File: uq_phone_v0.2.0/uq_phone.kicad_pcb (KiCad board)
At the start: 4 copper layers, 42.8 x 103.8 mm, 146 parts, among them J1 USB4105-GF-A, J10 SJ-3551B-MSMT-TR-67, J11 Conn_01x02, J2 BM03B-ACHSS-GAN-TF_LF__SN_, J3 20279-001E-03, J4 20279-001E-03, J5 6871XX14022_68715014022, J6 Conn_ARM_SWD_TagConnect_TC2030, J7 Conn_01x02, J8 KP15B-6S-SF_800_, M1 VCDM0834B004L, Q1 MMBT3904LP-7, Q2 MMBT3904LP-7, U1 MCP73871-2CCI_ML, U10 TPD3F303DQDR, U11 TPD8F003DQDR, U12 MCP1664T-E/OT, U13 TS3A5018RSVR, U14 NAU88C22YG, U2 TPS62162DSGR, U3 BQ27441DRZR-G1A, U4 WP SNAP-IN BASE_6000636, U5 TXB0108RGYR, U6 TXB0108RGYR, U7 STM32H733VGTx, U8 LSM6DSVTR, U9 DRV2603RUNR

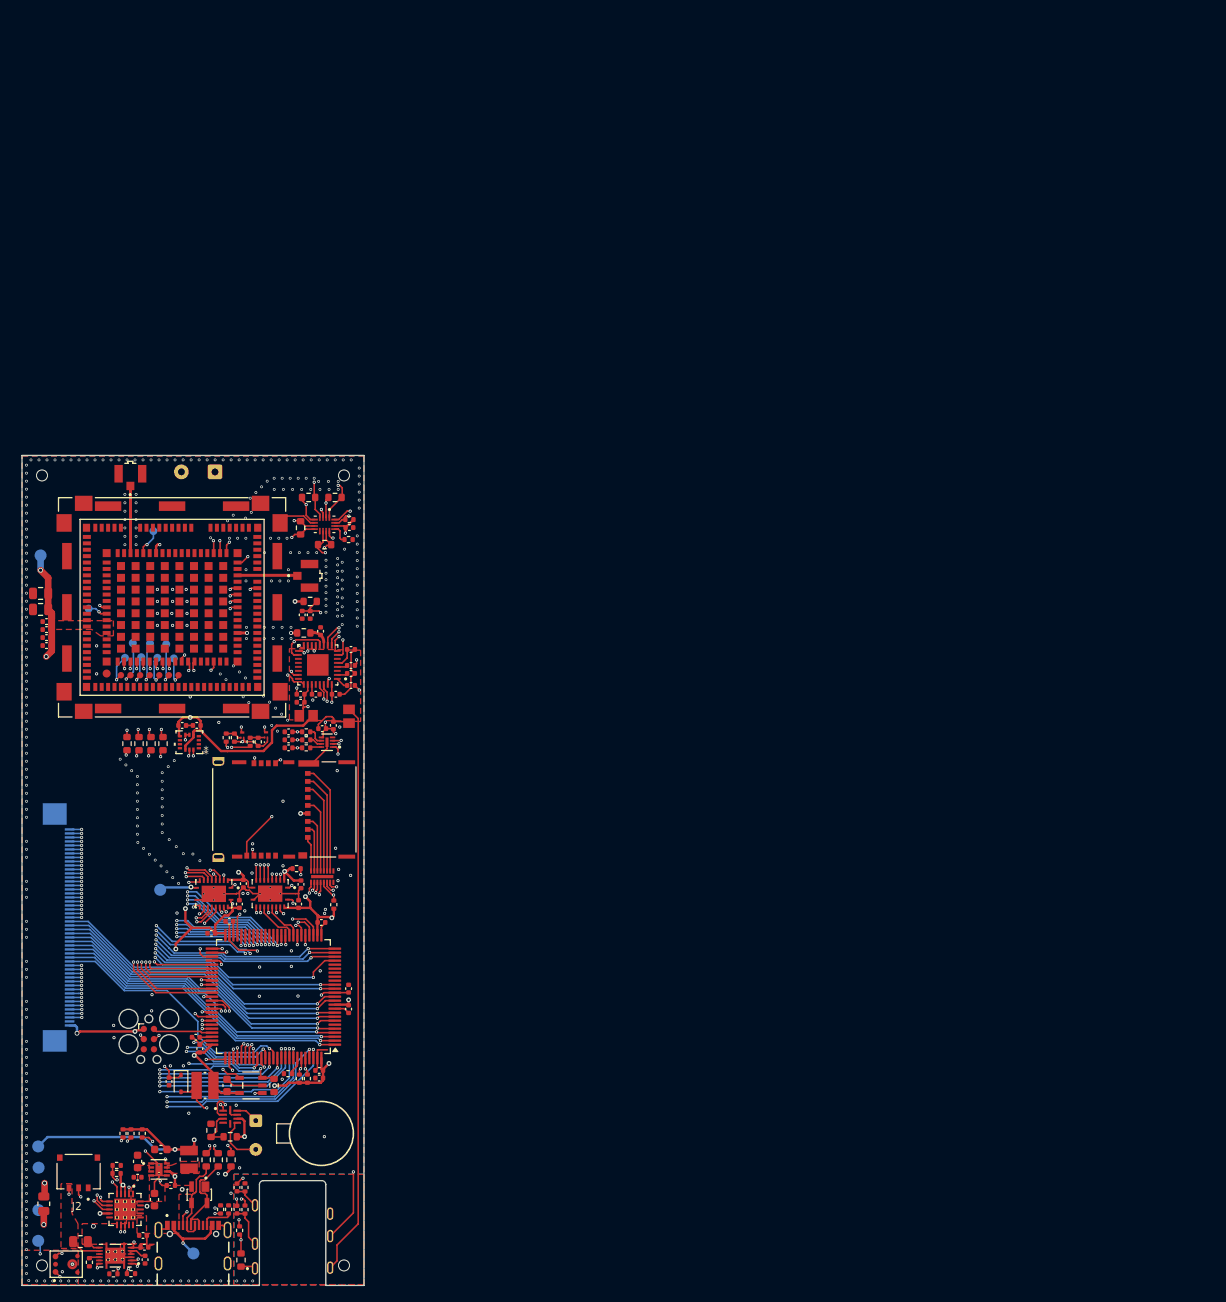
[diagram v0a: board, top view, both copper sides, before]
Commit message: Clean repo
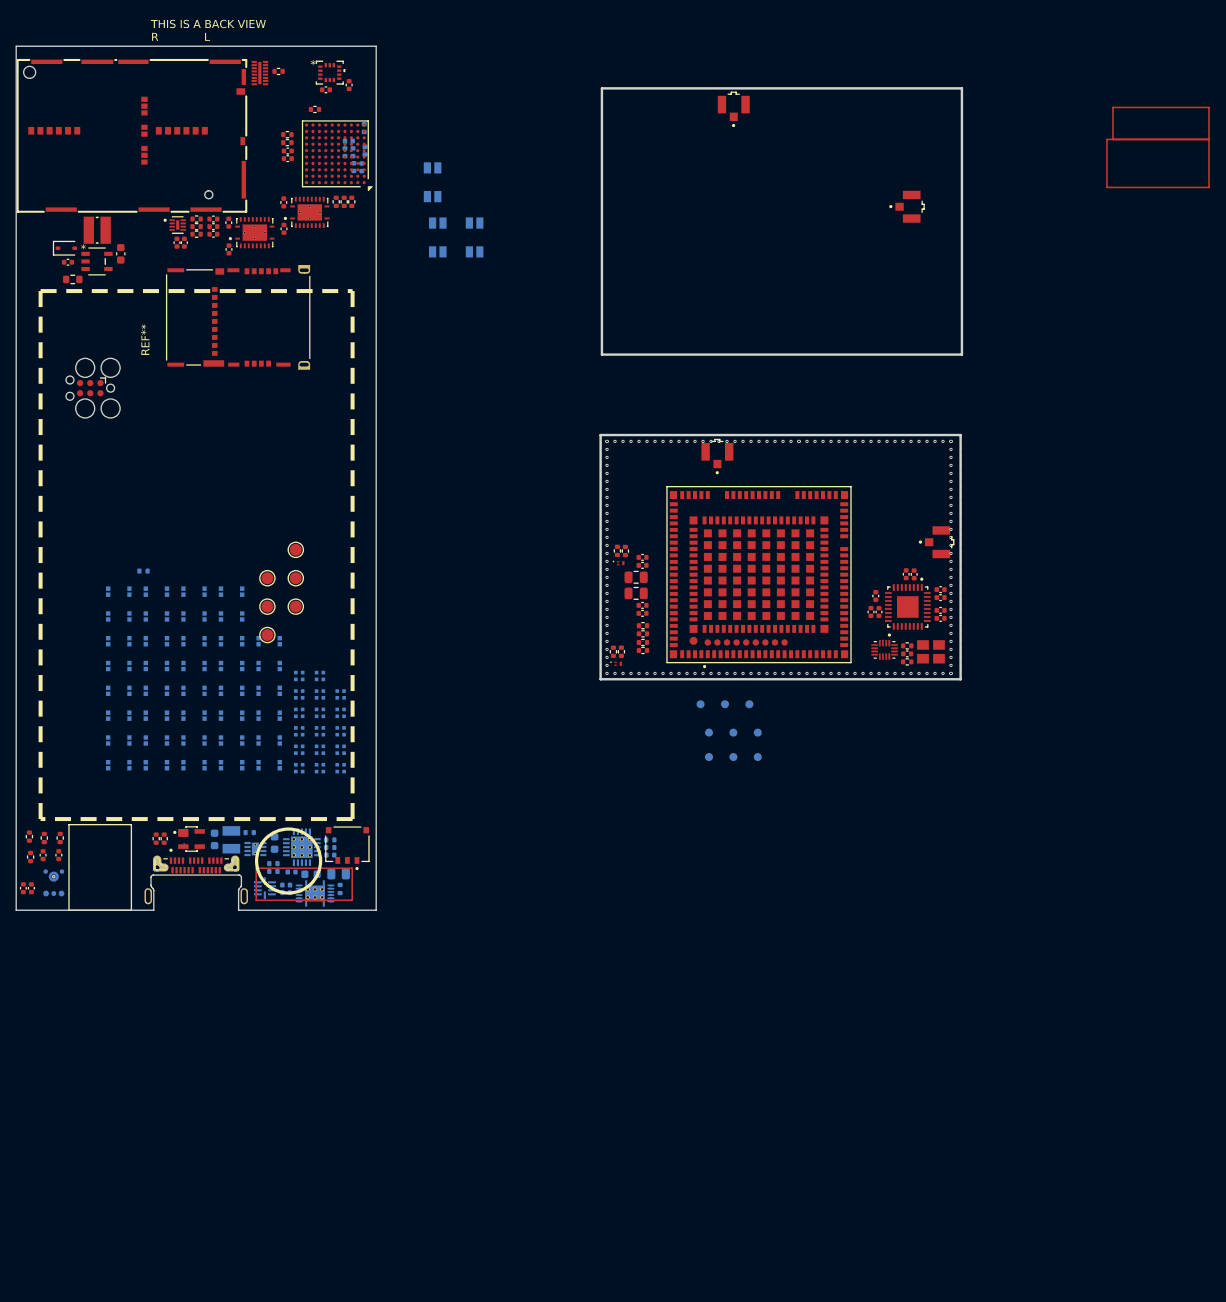
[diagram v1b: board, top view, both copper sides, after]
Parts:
- removed J1: USB4105-GF-A, USB_C_connector:GCT_USB4105-GF-A
- removed J10: SJ-3551B-MSMT-TR-67, SJ-3551B-MSMT-TR-67:CUI_SJ-3551B-MSMT-TR-67
- removed J11: Conn_01x02, Connector_Wire:SolderWire-0.25sqmm_1x02_P4.2mm_D0.65mm_OD1.7mm
- removed the J4 at (63.3, 83.3)
- removed the J5 at (31.0, 127.2)
- removed J7: Conn_01x02, Connector_Wire:SolderWire-0.1sqmm_1x02_P3.6mm_D0.4mm_OD1mm
- removed M1: VCDM0834B004L, custom_footprints:Motor_8mm
- removed R30, R31: 22R, Resistor_SMD:R_0402_1005Metric
- removed R34: 3.83R, Resistor_SMD:R_0603_1608Metric
- removed R35, R44, R49: 10k, Resistor_SMD:R_0402_1005Metric
- removed R37, R41, R43, R46, R47: 0R, Resistor_SMD:R_0603_1608Metric
- removed R4: 100k, Resistor_SMD:R_0402_1005Metric
- removed R45: 47k, Resistor_SMD:R_0402_1005Metric
- removed TP1: TestPoint, TestPoint:TestPoint_Pad_D1.5mm
- added J4: 20279-001E-03, 20279-001E-03:IPEX_20279-001E-03, F.Cu at (116.3, 24.4)
- added J4: 20279-001E-03, 20279-001E-03:IPEX_20279-001E-03, F.Cu at (114.3, 67.8)
- added J5: 20279-001E-03, 20279-001E-03:IPEX_20279-001E-03, F.Cu at (138.6, 37.2)
- added J5: 20279-001E-03, 20279-001E-03:IPEX_20279-001E-03, F.Cu at (142.3, 79.1)
- added LED1: XL-1010RGBC, custom_footprints:XL-1010RGBC-WS2812B, B.Cu at (62.0, 107.3)
- added LED10: XL-1010RGBC, custom_footprints:XL-1010RGBC-WS2812B, B.Cu at (64.6, 100.4)
- added LED11: XL-1010RGBC, custom_footprints:XL-1010RGBC-WS2812B, B.Cu at (64.6, 98.1)
- added LED12: XL-1010RGBC, custom_footprints:XL-1010RGBC-WS2812B, B.Cu at (64.6, 95.8)
- added LED13: XL-1010RGBC, custom_footprints:XL-1010RGBC-WS2812B, B.Cu at (67.2, 107.3)
- added LED14: XL-1010RGBC, custom_footprints:XL-1010RGBC-WS2812B, B.Cu at (67.2, 105.0)
- added LED15: XL-1010RGBC, custom_footprints:XL-1010RGBC-WS2812B, B.Cu at (67.2, 102.7)
- added LED16: XL-1010RGBC, custom_footprints:XL-1010RGBC-WS2812B, B.Cu at (67.2, 100.4)
- added LED17: XL-1010RGBC, custom_footprints:XL-1010RGBC-WS2812B, B.Cu at (67.2, 98.1)
- added LED2: XL-1010RGBC, custom_footprints:XL-1010RGBC-WS2812B, B.Cu at (62.0, 105.0)
- added LED3: XL-1010RGBC, custom_footprints:XL-1010RGBC-WS2812B, B.Cu at (62.0, 102.7)
- added LED4: XL-1010RGBC, custom_footprints:XL-1010RGBC-WS2812B, B.Cu at (62.0, 100.4)
- added LED5: XL-1010RGBC, custom_footprints:XL-1010RGBC-WS2812B, B.Cu at (62.0, 98.1)
- added LED6: XL-1010RGBC, custom_footprints:XL-1010RGBC-WS2812B, B.Cu at (62.0, 95.8)
- added LED7: XL-1010RGBC, custom_footprints:XL-1010RGBC-WS2812B, B.Cu at (64.6, 107.3)
- added LED8: XL-1010RGBC, custom_footprints:XL-1010RGBC-WS2812B, B.Cu at (64.6, 105.0)
- added LED9: XL-1010RGBC, custom_footprints:XL-1010RGBC-WS2812B, B.Cu at (64.6, 102.7)
- added R23: 10k, Resistor_SMD:R_0402_1005Metric, F.Cu at (60.5, 28.1)
- added REF**: HIROSE_KP15B-6S-SF_800_, KP15B-6S-SF_800_:HIROSE_KP15B-6S-SF_800_, F.Cu at (54.4, 51.0)
- added SW1: SKTAAAE010, custom_footprints:SKTAAAE010, B.Cu at (39.5, 107.0)
- added SW10: SKTAAAE010, custom_footprints:SKTAAAE010, B.Cu at (44.1, 107.0)
- added SW11: SKTAAAE010, custom_footprints:SKTAAAE010, B.Cu at (44.1, 103.8)
- added SW12: SKTAAAE010, custom_footprints:SKTAAAE010, B.Cu at (44.1, 100.8)
- added SW13: SKTAAAE010, custom_footprints:SKTAAAE010, B.Cu at (44.1, 97.7)
- added SW14: SKTAAAE010, custom_footprints:SKTAAAE010, B.Cu at (44.1, 94.5)
- added SW15: SKTAAAE010, custom_footprints:SKTAAAE010, B.Cu at (44.1, 91.5)
- added SW16: SKSCLCE010, custom_footprints:SKSCLCE010, B.Cu at (79.3, 41.0)
- added SW17: SKTAAAE010, custom_footprints:SKTAAAE010, B.Cu at (44.1, 88.3)
- added SW18: SKTAAAE010, custom_footprints:SKTAAAE010, B.Cu at (44.1, 85.2)
- added SW19: SKTAAAE010, custom_footprints:SKTAAAE010, B.Cu at (48.9, 107.0)
- added SW2: SKTAAAE010, custom_footprints:SKTAAAE010, B.Cu at (39.5, 103.8)
- added SW20: SKTAAAE010, custom_footprints:SKTAAAE010, B.Cu at (48.9, 103.8)
- added SW21: SKTAAAE010, custom_footprints:SKTAAAE010, B.Cu at (48.9, 100.8)
- added SW22: SKSCLCE010, custom_footprints:SKSCLCE010, B.Cu at (84.0, 41.0)
- added SW23: SKTAAAE010, custom_footprints:SKTAAAE010, B.Cu at (48.9, 97.7)
- added SW24: SKTAAAE010, custom_footprints:SKTAAAE010, B.Cu at (48.9, 94.5)
- added SW25: SKTAAAE010, custom_footprints:SKTAAAE010, B.Cu at (48.9, 91.5)
- added SW26: SKTAAAE010, custom_footprints:SKTAAAE010, B.Cu at (48.9, 88.3)
- added SW27: SKTAAAE010, custom_footprints:SKTAAAE010, B.Cu at (48.9, 85.2)
- added SW28: SKTAAAE010, custom_footprints:SKTAAAE010, B.Cu at (53.5, 107.0)
- added SW29: SKTAAAE010, custom_footprints:SKTAAAE010, B.Cu at (53.5, 103.8)
- added SW3: SKTAAAE010, custom_footprints:SKTAAAE010, B.Cu at (39.5, 100.8)
- added SW30: SKTAAAE010, custom_footprints:SKTAAAE010, B.Cu at (53.5, 100.8)
- added SW31: SKTAAAE010, custom_footprints:SKTAAAE010, B.Cu at (53.5, 97.7)
- added SW32: SKTAAAE010, custom_footprints:SKTAAAE010, B.Cu at (53.5, 94.5)
- added SW33: SKTAAAE010, custom_footprints:SKTAAAE010, B.Cu at (53.5, 91.5)
- added SW34: SKTAAAE010, custom_footprints:SKTAAAE010, B.Cu at (53.5, 88.3)
- added SW35: SKTAAAE010, custom_footprints:SKTAAAE010, B.Cu at (53.5, 85.2)
- added SW36: SKTAAAE010, custom_footprints:SKTAAAE010, B.Cu at (58.2, 107.0)
- added SW37: SKTAAAE010, custom_footprints:SKTAAAE010, B.Cu at (58.2, 103.8)
- added SW38: SKTAAAE010, custom_footprints:SKTAAAE010, B.Cu at (58.2, 100.8)
- added SW39: SKTAAAE010, custom_footprints:SKTAAAE010, B.Cu at (58.2, 97.7)
- added SW4: SKTAAAE010, custom_footprints:SKTAAAE010, B.Cu at (39.5, 97.7)
- added SW40: SKTAAAE010, custom_footprints:SKTAAAE010, B.Cu at (58.2, 94.5)
- added SW41: SKTAAAE010, custom_footprints:SKTAAAE010, B.Cu at (58.2, 91.5)
- added SW5: SKTAAAE010, custom_footprints:SKTAAAE010, B.Cu at (39.5, 94.5)
- added SW6: SKSCLCE010, custom_footprints:SKSCLCE010, B.Cu at (78.7, 34.1)
- added SW7: SKTAAAE010, custom_footprints:SKTAAAE010, B.Cu at (39.5, 91.5)
- added SW8: SKTAAAE010, custom_footprints:SKTAAAE010, B.Cu at (39.5, 88.3)
- added SW9: SKTAAAE010, custom_footprints:SKTAAAE010, B.Cu at (39.5, 85.2)
- C1, C15, C16, C17, C18, C5, C6, L1, MK1, R11, U3: moved to B.Cu
- C14: value 100nF -> 4.7uF; moved to B.Cu
- C19: value 4.7uF -> 100nF; moved to B.Cu
- C2: value 4.7uF -> 22uF; footprint Capacitor_SMD:C_0402_1005Metric -> Capacitor_SMD:C_0603_1608Metric; moved to B.Cu
- C20: value 2.2uF -> 100nF; moved to B.Cu
- C21: value 2.2uF -> 100nF
- C25, C26: value 100nF -> 2.2uF
- C27: value 100nF -> 10uF; footprint Capacitor_SMD:C_0402_1005Metric -> Capacitor_SMD:C_0603_1608Metric
- C28, C36: value 100nF -> 4.7uF
- C3: value 4.7uF -> 10uF; footprint Capacitor_SMD:C_0402_1005Metric -> Capacitor_SMD:C_0603_1608Metric; moved to B.Cu
- C34: value 10uF -> 100nF; footprint Capacitor_SMD:C_0603_1608Metric -> Capacitor_SMD:C_0402_1005Metric
- C35: value 4.7uF -> 100nF
- C38: value 1uF -> 100nF
- C39, C41, C43: value 1uF -> 4.7uF
- C4: value 10uF -> 4.7uF; footprint Capacitor_SMD:C_0603_1608Metric -> Capacitor_SMD:C_0402_1005Metric; moved to B.Cu
- C40: value 33pF -> 4.7uF
- C45, C47, C48, C49: value 4.7uF -> 1uF
- C46: value 4.7uF -> 33pF
- C7: value 22uF -> 4.7uF; footprint Capacitor_SMD:C_0603_1608Metric -> Capacitor_SMD:C_0402_1005Metric; moved to B.Cu
- J2: value BM03B-ACHSS-GAN-TF_LF__SN_ -> 124018312112A; footprint BM03B-ACHSS-GAN-TF_LF__SN_:JST_BM03B-ACHSS-GAN-TF_LF__SN_ -> 124018312112A:AMPHENOL_124018312112A
- J3: value 20279-001E-03 -> BM03B-ACHSS-GAN-TF_LF__SN_; footprint 20279-001E-03:IPEX_20279-001E-03 -> BM03B-ACHSS-GAN-TF_LF__SN_:JST_BM03B-ACHSS-GAN-TF_LF__SN_
- J8: value KP15B-6S-SF_800_ -> MCS-302S-C1; footprint KP15B-6S-SF_800_:HIROSE_KP15B-6S-SF_800_ -> custom_footprints:SIM-SMD_MCS-302S-C1
- R1: value 270k -> 100k; moved to B.Cu
- R10: value 0R -> 2.2k; footprint Resistor_SMD:R_0805_2012Metric -> Resistor_SMD:R_0402_1005Metric; moved to B.Cu
- R12: value 4.7k -> 0R
- R13: value 47k -> 0R
- R14, R15: footprint Resistor_SMD:R_0603_1608Metric -> Resistor_SMD:R_0402_1005Metric
- R16, R21, R22: value 0R -> 4.7k; footprint Resistor_SMD:R_0603_1608Metric -> Resistor_SMD:R_0402_1005Metric
- R19: value 0R -> 47k; footprint Resistor_SMD:R_0603_1608Metric -> Resistor_SMD:R_0402_1005Metric
- R2: value 100k -> 5.1k
- R20, R40: value 0R -> 10k; footprint Resistor_SMD:R_0603_1608Metric -> Resistor_SMD:R_0402_1005Metric
- R24, R25: value 4.7k -> 10k
- R26, R27: value 10k -> 22R
- R28: value 0R -> 22R; footprint Resistor_SMD:R_0603_1608Metric -> Resistor_SMD:R_0402_1005Metric
- R29: value 0R -> 3.83R
- R3: value 2.2k -> 5.1k
- R32: value 22R -> 10k
- R36: value 10k -> 2.2k
- R38: value 2.2k -> 47k
- R42: value 0R -> 330R; footprint Resistor_SMD:R_0603_1608Metric -> Resistor_SMD:R_0402_1005Metric; moved to B.Cu
- R5: value 5.1k -> 270k; moved to B.Cu
- R7: value 10k -> 100k; moved to B.Cu
- R8: value 10m -> 10k; footprint Resistor_SMD:R_0805_2012Metric -> Resistor_SMD:R_0402_1005Metric; moved to B.Cu
- R9: value 5.1k -> 10m; footprint Resistor_SMD:R_0402_1005Metric -> Resistor_SMD:R_0805_2012Metric; moved to B.Cu
- TP2, TP3, TP4, TP5, TP6, TP7: moved to F.Cu
- U1: value MCP73871-2CCI_ML -> TPS62162DSGR; footprint MCP73871-2CCI_ML:QFN50P400X400X100-21N -> TPS62162DSGR:SON50P200X200X80-9N; moved to B.Cu
- U10: value TPD3F303DQDR -> TPD8F003DQDR; footprint TPD3F303DQDR:SON40P170X135X80-9N -> TPD8F003DQDR:SON40P135X330X80-17N
- U11: value TPD8F003DQDR -> LSM6DSVTR; footprint TPD8F003DQDR:SON40P135X330X80-17N -> LSM6DSVTR:LGA14-L_2P59X3P1X0P5_STM
- U12: value MCP1664T-E/OT -> DRV2603RUNR; footprint MCP1664T_E_OT:SOT-23-5_OT_MCH -> DRV2603RUNR:QFN50P200X200X80-10N; moved to B.Cu
- U2: value TPS62162DSGR -> MCP73871-2CCI_ML; footprint TPS62162DSGR:SON50P200X200X80-9N -> MCP73871-2CCI_ML:QFN50P400X400X100-21N; moved to B.Cu
- U4: footprint WP_SNAP-IN_BASE:SIERRA_WP_SNAP-IN_BASE -> RC7620_1104625:XCVR_RC7620_1104625
- U6: value TXB0108RGYR -> STM32H733VGHx; footprint TXB0108RGYR:IC_TXB0108RGYR -> Package_BGA:TFBGA-100_8x8mm_Layout10x10_P0.8mm
- U7: value STM32H733VGTx -> TXB0108RGYR; footprint Package_QFP:LQFP-100_14x14mm_P0.5mm -> TXB0108RGYR:IC_TXB0108RGYR
- U8: value LSM6DSVTR -> TPD3F303DQDR; footprint LSM6DSVTR:LGA14-L_2P59X3P1X0P5_STM -> TPD3F303DQDR:SON40P170X135X80-9N
- U9: value DRV2603RUNR -> MCP1664T-E/OT; footprint DRV2603RUNR:QFN50P200X200X80-10N -> MCP1664T_E_OT:SOT-23-5_OT_MCH
- moved R6 138.0 mm to (64.0, 25.0), turned to 180 degrees
- moved C34 126.0 mm to (68.3, 21.9), turned to -90 degrees
- moved R25 126.0 mm to (59.5, 20.2), turned to 0 degrees
- moved C35 125.5 mm to (65.4, 22.6), turned to 0 degrees
- moved R24 117.0 mm to (60.5, 29.1), turned to 180 degrees
- moved C39 116.6 mm to (142.2, 86.0), turned to 0 degrees
- moved C19 116.2 mm to (68.2, 28.9)
- moved C25 115.0 mm to (60.6, 31.1), turned to 180 degrees
- moved R27 114.7 mm to (49.2, 38.7), turned to 0 degrees
- moved R28 113.8 mm to (49.2, 39.6)
- moved C26 112.7 mm to (60.6, 30.2), turned to 180 degrees
- moved R26 112.7 mm to (49.2, 40.6), turned to 0 degrees
- moved U9 108.2 mm to (36.8, 44.0)
- moved R29 107.8 mm to (33.7, 46.2), turned to 0 degrees
- moved L2 107.7 mm to (36.8, 40.1)
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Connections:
- C1 pad 1: VUSB -> GND
- C1 pad 2: GND -> MCP_OUT
- C10 pad 1: +VMOB -> VBAT
- C11 pad 1: +VMOB -> VBAT
- C12 pad 1: +VMOB -> VBAT
- C13 pad 1: +VMOB -> VBAT
- C14 pad 1: +1.8V -> +3.3V
- C15 pad 1: +1.8V -> GND
- C15 pad 2: GND -> +3.3V
- C16 pad 1: +3.3V -> GND
- C16 pad 2: GND -> +3.3V
- C17 pad 1: +3.3V -> GND
- C17 pad 2: GND -> +3.3V
- C18 pad 2: RST -> +3.3V
- C19 pad 1: +3.3V -> GND
- C19 pad 2: GND -> +3.3V
- C2 pad 1: VBAT -> +3.3V
- C20 pad 1: Net-(C20-Pad1) -> GND
- C20 pad 2: GND -> RST
- C21 pad 1: Net-(C21-Pad1) -> +1.8V
- C22 pad 1: GND -> +3.3V
- C22 pad 2: +3.3V -> GND
- C23 pad 1: GND -> +1.8V
- C23 pad 2: +3.3V -> GND
- C24 pad 1: GND -> +3.3V
- C24 pad 2: +3.3V -> GND
- C25 pad 1: GND -> Net-(C25-Pad1)
- C25 pad 2: +3.3V -> GND
- C26 pad 1: GND -> Net-(C26-Pad1)
- C26 pad 2: +3.3V -> GND
- C28 pad 1: +3.3V -> DISP_LEDA
- C3 pad 1: MCP_OUT -> VUSB
- C35 pad 1: DISP_LEDA -> +3.3V
- C36 pad 1: +1.8V -> Net-(MK1-OUTPUT)
- C36 pad 2: GND -> MIC_OUT
- C37 pad 1: HP_MIC -> AGND
- C37 pad 2: Net-(C37-Pad2) -> MIC_GND
- C38 pad 1: HP_LEFT -> +1.8V
- C38 pad 2: Net-(C38-Pad2) -> GND
- C39 pad 1: HP_RIGHT -> Net-(U14-VDDA)
- C39 pad 2: Net-(C39-Pad2) -> AGND
- C4 pad 1: GND -> MCP_OUT
- C4 pad 2: MCP_OUT -> GND
- C40 pad 1: Net-(U14-MCLK) -> Net-(U14-VDDA)
- C40 pad 2: GND -> AGND
- C41 pad 1: Net-(U14-RMICN) -> +1.8V
- C41 pad 2: AGND -> GND
- C42 pad 1: Net-(MK1-OUTPUT) -> +1.8V
- C42 pad 2: MIC_OUT -> GND
- C43 pad 1: AGND -> Net-(U14-VREF)
- C43 pad 2: MIC_GND -> AGND
- C44 pad 1: Net-(U14-VDDB) -> MIC_BIAS
- C44 pad 2: GND -> AGND
- C45 pad 1: MIC_BIAS -> Net-(U14-RMICN)
- C46 pad 1: Net-(U14-VDDB) -> MOB_SYS_CLK
- C47 pad 1: Net-(U14-VDDA) -> Net-(U14-RMICP)
- C47 pad 2: AGND -> HP_MIC
- C48 pad 1: Net-(U14-VREF) -> HP_LEFT
- C48 pad 2: AGND -> Net-(C48-Pad2)
- C49 pad 1: Net-(U14-VDDA) -> HP_RIGHT
- C49 pad 2: AGND -> Net-(C49-Pad2)
- C7 pad 1: +3.3V -> VBAT
- C8 pad 1: +VMOB -> VBAT
- C9 pad 1: +VMOB -> VBAT
- FB1 pad 1: GND -> Net-(U14-VDDA)
- FB1 pad 2: AGND -> +3.3V
- FB2 pad 1: Net-(U14-VDDA) -> GND
- FB2 pad 2: +3.3V -> AGND
- J3 pad 1: MOB_MAIN_ANT -> GND
- J3 pad 2: GND -> BAT_THERM
- J3 pad 3: (no net) -> Net-(U3-BAT)
- L1 pad 1: Net-(U2-SW) -> Net-(U1-SW)
- R1 pad 1: Net-(U1-VPCC) -> Net-(U1-PG)
- R1 pad 2: VUSB -> +3.3V
- R10 pad 1: +VMOB -> Net-(U2-PROG1)
- R10 pad 2: VBAT -> GND
- R11 pad 1: Net-(U2-PG) -> GND
- R11 pad 2: +3.3V -> Net-(U2-PROG3)
- R12 pad 1: Net-(Q1-Pad1) -> Net-(U4A-UART1_TX)
- R12 pad 2: MOB_PWR_CTL -> MOB_TXD
- R13 pad 1: GND -> Net-(U4A-UART1_RTS)
- R13 pad 2: Net-(Q1-Pad1) -> MOB_RTS
- R14 pad 1: /Mobile/MOB_USB_N -> Net-(U4A-UART1_RX)
- R14 pad 2: USB_N -> MOB_RXD
- R15 pad 1: /Mobile/MOB_USB_P -> Net-(U4A-UART1_CTS)
- R15 pad 2: USB_P -> MOB_CTS
- R16 pad 1: Net-(U4A-USB_VBUS) -> Net-(Q1-Pad1)
- R16 pad 2: VUSB -> MOB_PWR_CTL
- R18 pad 2: Net-(Q2-Pad1) -> Net-(Q1-Pad1)
- R19 pad 1: Net-(U4A-UART1_TX) -> GND
- R19 pad 2: MOB_TXD -> Net-(Q2-Pad1)
- R2 pad 2: Net-(U1-VPCC) -> Net-(J2-CC1)
- R20 pad 1: Net-(U4A-UART1_RTS) -> GND
- R20 pad 2: MOB_RTS -> Net-(U6-BOOT0)
- R21 pad 1: Net-(U4A-UART1_RX) -> SCL
- R21 pad 2: MOB_RXD -> +3.3V
- R22 pad 1: Net-(U4A-UART1_CTS) -> SDA
- R22 pad 2: MOB_CTS -> +3.3V
- R24 pad 1: SCL -> MCP_STAT1
- R25 pad 1: SDA -> uSD_DET
- R26 pad 1: MCP_STAT2 -> Net-(U8-DATA2_IN)
- R26 pad 2: +3.3V -> SIM_DATA
- R27 pad 1: MCP_STAT1 -> Net-(U8-DATA1_IN)
- R27 pad 2: +3.3V -> SIM_RST
- R28 pad 1: Net-(U9-LRA/~{ERM}) -> Net-(U8-CLK_IN)
- R28 pad 2: +3.3V -> SIM_CLK
- R29 pad 2: Net-(U9-LRA/~{ERM}) -> DISP_LEDK
- R3 pad 1: Net-(U1-PROG1) -> GND
- R3 pad 2: GND -> Net-(J2-CC2)
- R32 pad 1: Net-(U10-CLK_IN) -> AUD_SW_L
- R32 pad 2: SIM_CLK -> +1.8V
- R33 pad 1: uSD_DET -> GND
- R33 pad 2: +3.3V -> Net-(U13-~{EN})
- R36 pad 1: GND -> HP_MIC
- R36 pad 2: Net-(U13-~{EN}) -> MIC_BIAS
- R38 pad 1: Net-(C37-Pad2) -> HP_DET
- R38 pad 2: MIC_BIAS -> +1.8V
- R39 pad 1: Net-(C38-Pad2) -> Net-(C48-Pad2)
- R40 pad 1: MOB_AUD_SYNC -> Net-(C49-Pad2)
- R40 pad 2: AUD_SYNC -> AGND
- R42 pad 1: MOB_AUD_IN -> Net-(LED15-DI)
- R42 pad 2: AUD_IN -> LED_DATA
- R5 pad 1: GND -> Net-(U2-VPCC)
- R5 pad 2: Net-(J1-CC2) -> VUSB
- R6 pad 1: GND -> FUEL_GPO
- R6 pad 2: Net-(J1-CC1) -> +3.3V
- R7 pad 2: Net-(U3-BIN) -> Net-(U2-VPCC)
- R8 pad 1: Net-(U3-BAT) -> GND
- R8 pad 2: VBAT -> Net-(U3-BIN)
- R9 pad 1: FUEL_GPO -> Net-(U3-BAT)
- R9 pad 2: +3.3V -> VBAT
- TP2 pad 1: GND -> VUSB
- TP4 pad 1: AGND -> VBAT
- TP5 pad 1: VBAT -> +1.8V
- TP6 pad 1: +VMOB -> GND
- TP7 pad 1: +1.8V -> AGND
- TP8 pad 1: Net-(U4A-TP1_BOOTPIN) -> Net-(U4A-TX_ON)
- TP9 pad 1: Net-(U4A-TX_ON) -> Net-(U4A-TP1_BOOTPIN)
- U1 pad 1: MCP_OUT -> GND
- U1 pad 2: Net-(U1-VPCC) -> MCP_OUT
- U1 pad 3: VUSB -> MCP_OUT
- U1 pad 4: VUSB -> GND
- U1 pad 5: BAT_THERM -> GND
- U1 pad 6: MCP_PG -> +3.3V
- U1 pad 7: MCP_STAT2 -> Net-(U1-SW)
- U1 pad 8: MCP_STAT1 -> Net-(U1-PG)
- U1 pad 9: VUSB -> GND
- U10 pad 1: Net-(J8B-RST) -> uSD_DAT2
- U10 pad 2: Net-(J8B-CLK_2) -> uSD_DAT3
- U10 pad 3: Net-(J8B-I/O) -> uSD_CMD
- U10 pad 4: (no net) -> uSD_CLK
- U10 pad 5: SIM_VDD -> uSD_DET
- U10 pad 6: Net-(U10-DATA2_IN) -> uSD_DAT0
- U10 pad 7: Net-(U10-CLK_IN) -> uSD_DAT1
- U10 pad 8: Net-(U10-DATA1_IN) -> unconnected-(U10-CH8_IN-Pad8)
- U10 pad 9: GND -> unconnected-(U10-CH8_OUT-Pad9)
- U11 pad 1: uSD_DAT2 -> GND
- U11 pad 10: Net-(J8A-DAT1) -> unconnected-(U11-OCS_AUX-Pad10)
- U11 pad 11: Net-(J8A-DAT0) -> unconnected-(U11-SDO_AUX-Pad11)
- U11 pad 12: Net-(U11-CH5_OUT) -> +3.3V
- U11 pad 13: Net-(J8A-CLK) -> SCL
- U11 pad 14: Net-(J8A-CMD) -> SDA
- U11 pad 2: uSD_DAT3 -> GND
- U11 pad 3: uSD_CMD -> GND
- U11 pad 4: uSD_CLK -> unconnected-(U11-INT1-Pad4)
- U11 pad 5: uSD_DET -> +3.3V
- U11 pad 6: uSD_DAT0 -> GND
- U11 pad 7: uSD_DAT1 -> GND
- U11 pad 8: unconnected-(U11-CH8_IN-Pad8) -> +3.3V
- U12 pad 1: Net-(D2-A) -> VIB_EN
- U12 pad 2: GND -> VIB_PWM
- U12 pad 3: DISP_LEDK -> GND
- U12 pad 4: DISP_BL -> (no net)
- U12 pad 5: +3.3V -> GND
- U14 pad 11: Net-(U14-MCLK) -> MOB_SYS_CLK
- U14 pad 13: Net-(U14-VDDB) -> +1.8V
- U14 pad 14: Net-(U14-VDDB) -> +1.8V
- U14 pad 4: HP_MIC -> Net-(U14-RMICP)
- U2 pad 1: GND -> MCP_OUT
- U2 pad 2: MCP_OUT -> Net-(U2-VPCC)
- U2 pad 3: MCP_OUT -> VUSB
- U2 pad 4: GND -> VUSB
- U2 pad 5: GND -> BAT_THERM
- U2 pad 6: +3.3V -> MCP_PG
- U2 pad 7: Net-(U2-SW) -> MCP_STAT2
- U2 pad 8: Net-(U2-PG) -> MCP_STAT1
- U2 pad 9: GND -> VUSB
- U4 pad 12: /Mobile/MOB_USB_N -> unconnected-(U4A-USB_D--Pad12)
- U4 pad 13: /Mobile/MOB_USB_P -> unconnected-(U4A-USB_D+-Pad13)
- U4 pad 157: +VMOB -> VBAT
- U4 pad 158: +VMOB -> VBAT
- U4 pad 16: Net-(U4A-USB_VBUS) -> unconnected-(U4A-USB_VBUS-Pad16)
- U4 pad 61: +VMOB -> VBAT
- U4 pad 62: +VMOB -> VBAT
- U4 pad 63: +VMOB -> VBAT
- U7 pad 1: PB_HASH -> AUD_SDA
- U7 pad 10: GND -> +1.8V
- U7 pad 11: +3.3V -> GND
- U7 pad 12: PB_8 -> MCU_AUD_OUT_L_H
- U7 pad 13: PB_9 -> MCU_AUD_BCLK_H
- U7 pad 14: RST -> AUD_SW_H
- U7 pad 15: PB_MENU_L -> MCU_AUD_SYNC_H
- U7 pad 16: PB_MENU_R -> HP_DET_MCU
- U7 pad 17: unconnected-(U7-PC2_C-Pad17) -> MOB_WAKE_H
- U7 pad 18: unconnected-(U7-PC3_C-Pad18) -> SCL
- U7 pad 19: GND -> +3.3V
- U7 pad 2: PB_1 -> +1.8V
- U7 pad 20: unconnected-(U7-VREF+-Pad20) -> SDA
- U7 pad 21: unconnected-(U7-VDDA-Pad21) -> GND
- U7 pad 3: PB_2 -> AUD_SCL
- U7 pad 4: PB_3 -> MOB_WAKE_L
- U7 pad 5: PB_4 -> HP_DET
- U7 pad 6: unconnected-(U7-VBAT-Pad6) -> MCU_AUD_SYNC_L
- U7 pad 7: PB_5 -> AUD_SW_L
- U7 pad 8: PB_6 -> MCU_AUD_BCLK_L
- U7 pad 9: PB_7 -> MCU_AUD_OUT_L
- U8 pad 1: GND -> Net-(J8B-SIM_1_RST)
- U8 pad 2: GND -> Net-(J8B-SIM_1_CLK)
- U8 pad 3: GND -> Net-(J8B-SIM_1_DATA)
- U8 pad 4: unconnected-(U8-INT1-Pad4) -> (no net)
- U8 pad 5: +3.3V -> SIM_VDD
- U8 pad 6: GND -> Net-(U8-DATA2_IN)
- U8 pad 7: GND -> Net-(U8-CLK_IN)
- U8 pad 8: +3.3V -> Net-(U8-DATA1_IN)
- U8 pad 9: unconnected-(U8-INT2-Pad9) -> GND
- U9 pad 1: VIB_EN -> Net-(D2-A)
- U9 pad 2: VIB_PWM -> GND
- U9 pad 3: Net-(U9-LRA/~{ERM}) -> DISP_LEDK
- U9 pad 4: (no net) -> DISP_BL
- U9 pad 5: GND -> +3.3V
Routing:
- net +3.3V: track 246.4 -> 0.00 mm, vias 16 -> 0
- net +1.8V: track 115.8 -> 0.00 mm, vias 6 -> 0
- net AGND: track 111.9 -> 0.00 mm, vias 5 -> 0
- net Net-(MK1-OUTPUT): track 109.6 -> 0.00 mm, vias 2 -> 0
- net MIC_BIAS: track 106.3 -> 0.00 mm, vias 3 -> 0
- net SDA: track 91.7 -> 0.00 mm, vias 6 -> 0
- net SCL: track 91.6 -> 0.00 mm, vias 6 -> 0
- net HP_DET: track 89.6 -> 0.00 mm, vias 5 -> 0
- net +VMOB: track 81.8 -> 0.00 mm, vias 3 -> 0
- net GND: track 81.8 -> 0.00 mm, vias 375 -> 148
- net Net-(C37-Pad2): track 81.7 -> 0.00 mm, vias 2 -> 0
- net HP_RIGHT: track 78.2 -> 0.00 mm, vias 2 -> 0
- net HP_LEFT: track 75.5 -> 0.00 mm, vias 2 -> 0
- net Net-(U4A-USB_VBUS): track 63.0 -> 0.00 mm, vias 2 -> 0
- net /Mobile/MOB_USB_N: track 63.0 -> 0.00 mm, vias 2 -> 0
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- added copper zone on In3.Cu, net GND
- added copper zone on In4.Cu, net GND
- removed copper zone on F.Cu, net +VMOB
- removed copper zone on B.Cu, net AGND
- removed copper zone on F.Cu, net AGND
- removed copper zone on F.Cu, net MCP_OUT
- removed copper zone on F.Cu, net Net-(U2-SW)
- removed copper zone on F.Cu, net Net-(U3-BAT)
- removed copper zone on F.Cu, net VBAT
- removed copper zone on F.Cu, net VUSB
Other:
- board size 42.8 x 103.8 mm -> 118.2 x 108 mm
- copper layers 4 -> 6
- board text added: "Battery"
- board text added: "Non Socket Version"
- board text added: "Socket Version"
- board text added: "THIS IS A BACK VIEW R L"
- board text removed: "LEFT"
- board text removed: "RIGHT"
